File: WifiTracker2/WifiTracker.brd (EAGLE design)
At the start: 78.7 x 50.5 mm, 27 parts, among them Y1 16MHz

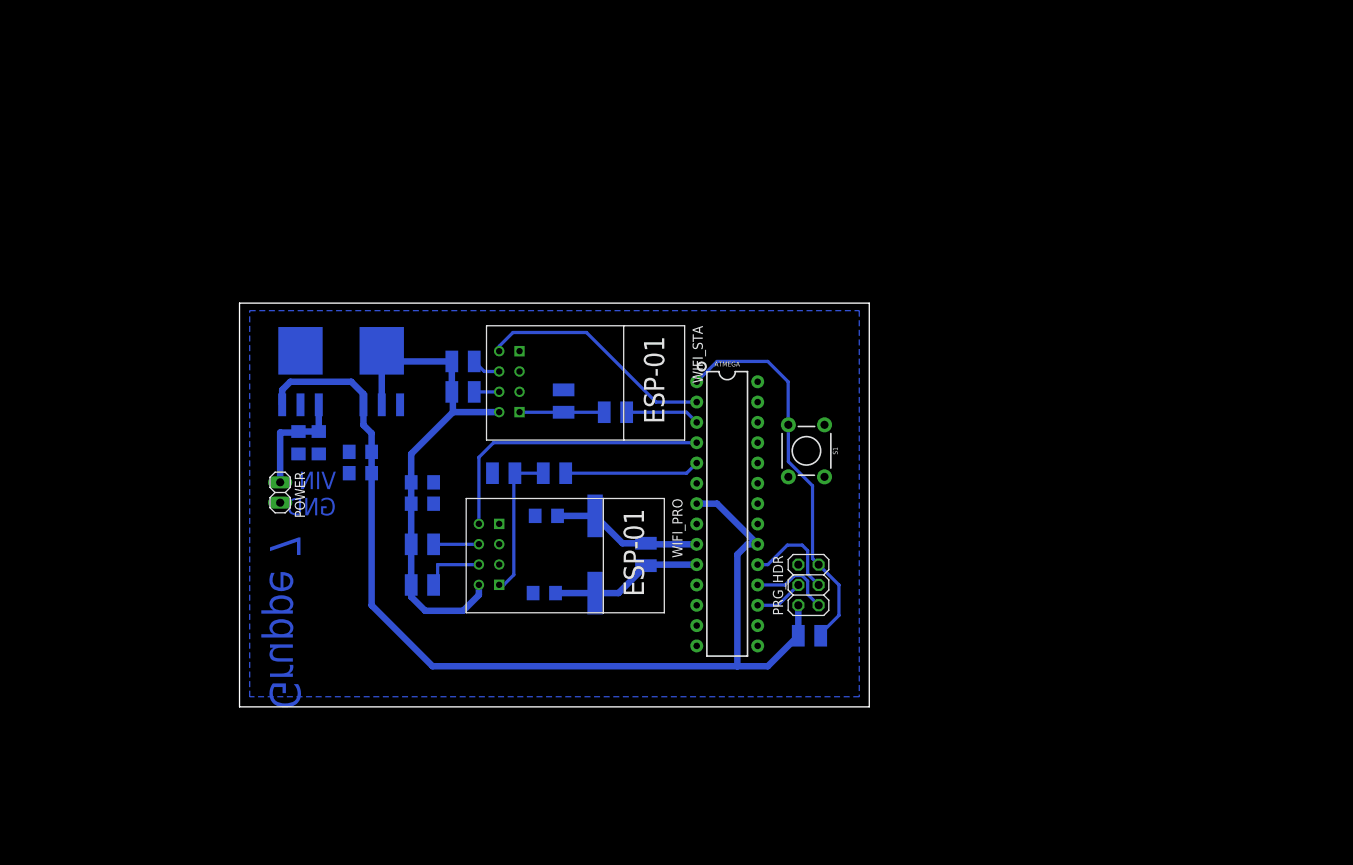
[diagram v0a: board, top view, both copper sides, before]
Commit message: update
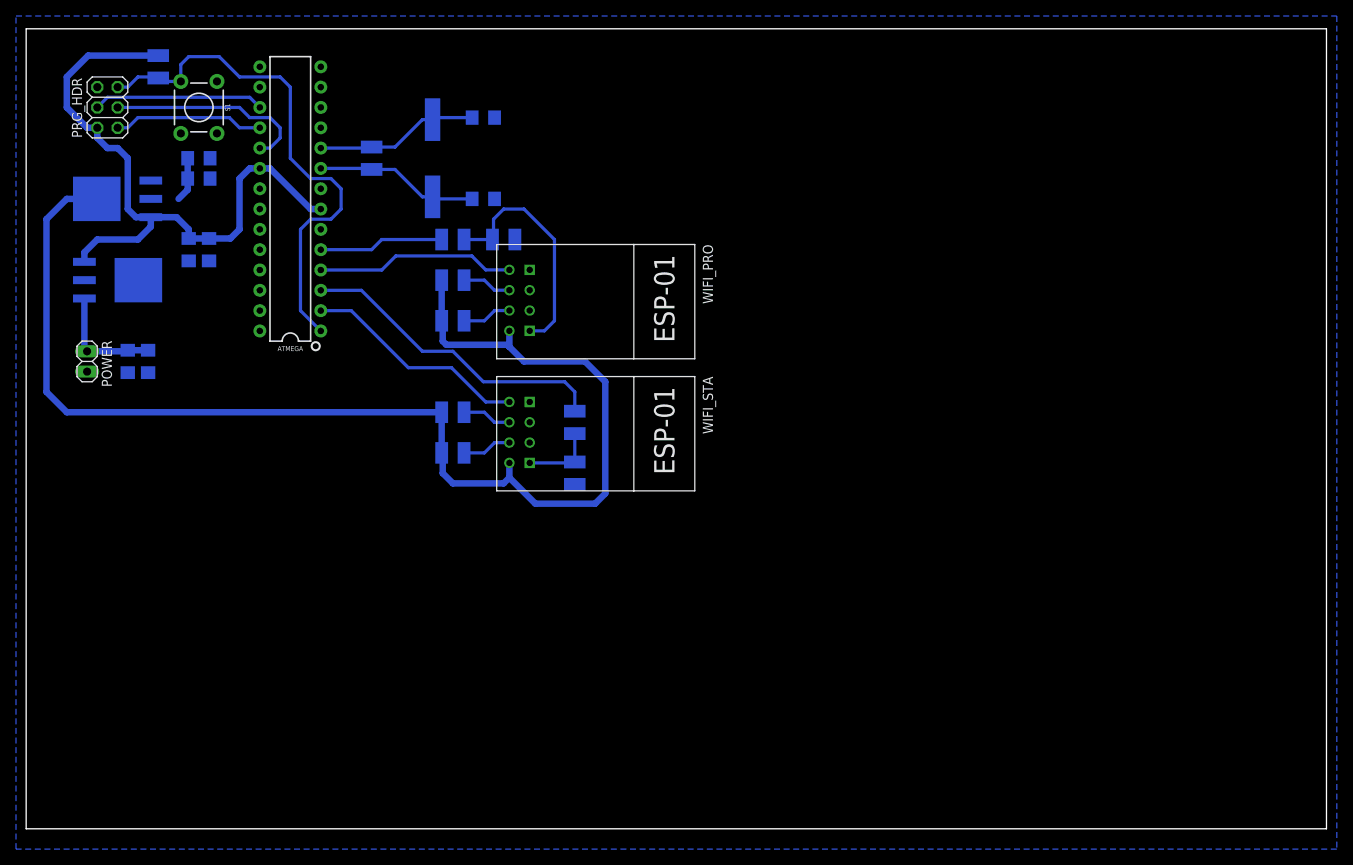
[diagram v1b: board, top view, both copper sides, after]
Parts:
- moved R6 108.1 mm to (14.0, 95.2), turned to 270 degrees
- moved PRG_HDR 106.0 mm to (7.62, 90.2)
- moved S1 87.2 mm to (19.1, 90.2)
- moved ATMEGA 67.3 mm to (30.5, 78.7), turned to 90 degrees
- moved R4 60.2 mm to (40.6, 83.8), turned to 270 degrees
- moved C2 59.9 mm to (54.6, 88.9), turned to 0 degrees
- moved Y1 53.5 mm to (48.3, 83.8), turned to 270 degrees
- moved C6 49.3 mm to (19.1, 81.3)
- moved C9 49.2 mm to (19.1, 83.8)
- moved C1 40.4 mm to (54.6, 78.7), turned to 0 degrees
- moved 3V_REG 39.5 mm to (8.89, 78.7), turned to 0 degrees
- moved C8 35.2 mm to (17.8, 72.4), turned to 270 degrees
- moved R3 33.2 mm to (50.8, 68.6)
- moved R5 33.2 mm to (50.8, 63.5)
- moved WIFI_PRO 32.0 mm to (66.0, 66.0)
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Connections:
- net 3VCC: no longer 3V_REG.2
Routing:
- net 3VCC: track 64.8 -> 163.5 mm
- net 5VCC: track 128.7 -> 81.6 mm
- net AT_TXD: track 9.29 -> 39.4 mm
- net ATMEGA_RESET: track 48.9 -> 65.8 mm
- net MOSI: track 6.13 -> 21.4 mm
- net SCK: track 12.4 -> 25.7 mm
- net PRO_TXD: track 36.3 -> 25.0 mm
- net PRO_RXD: track 18.7 -> 29.6 mm
- net MISO: track 10.6 -> 18.8 mm
- net STA_RST: track 3.12 -> 6.19 mm
- net STA_CH_PD: track 3.64 -> 6.18 mm
- net PRO_RST: track 8.20 -> 6.19 mm
- net XTAL1: track 18.9 -> 20.5 mm
- net XTAL2: track 19.1 -> 20.6 mm
- net STA_RXD: track 10.6 -> 9.24 mm
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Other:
- board size 78.7 x 50.5 mm -> 162.5 x 100 mm
- board text removed: "Gruppe 7"
- board text removed: "VIN GND"
